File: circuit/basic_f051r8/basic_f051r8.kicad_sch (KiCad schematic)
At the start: 1 part

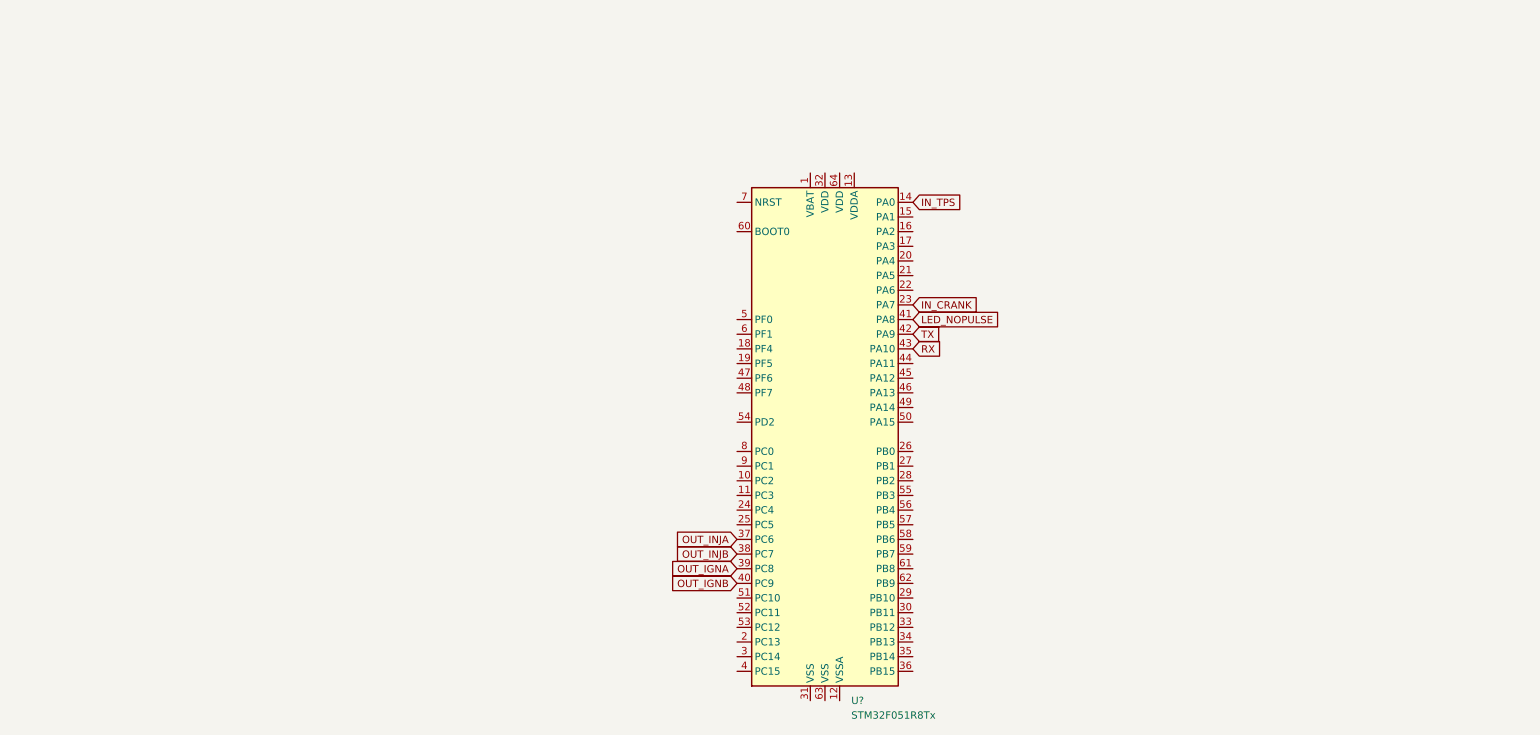
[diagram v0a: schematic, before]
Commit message: Schematic
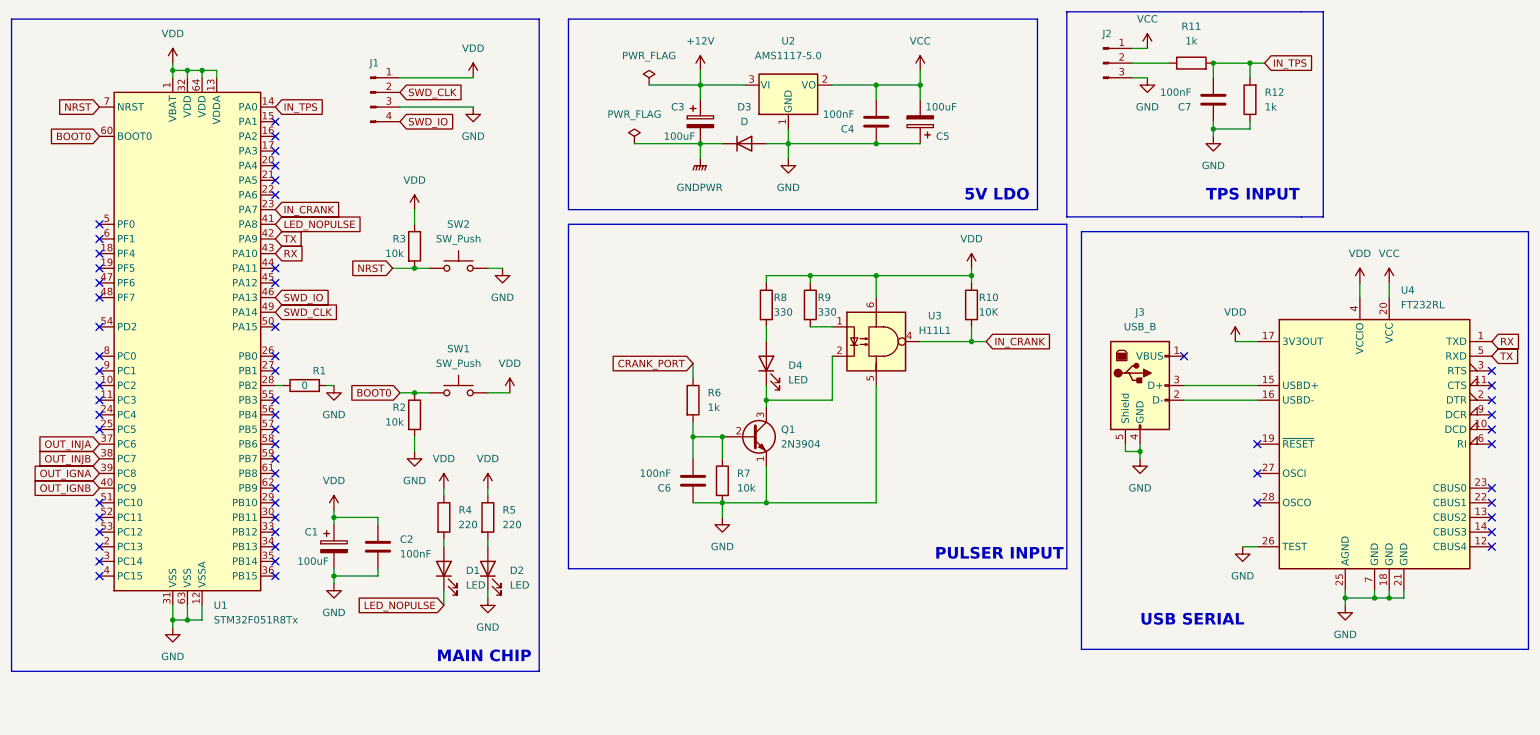
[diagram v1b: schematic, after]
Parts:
- added C1, C3, C5: 100uF, symbol Device:C_Polarized
- added C2, C4, C6, C7: 100nF, symbol Device:C
- added D1, D2, D4: LED, symbol Device:LED
- added D3: D, symbol Device:D
- added J1: Conn_01x04_Male, symbol Connector:Conn_01x04_Male
- added J2: Conn_01x03_Male, symbol Connector:Conn_01x03_Male
- added J3: USB_B, symbol Connector:USB_B
- added Q1: 2N3904, Package_TO_SOT_THT:TO-92_Inline, symbol Transistor_BJT:2N3904
- added R1: 0, symbol Device:R
- added R10: 10K, symbol Device:R
- added R11, R12, R6: 1k, symbol Device:R
- added R2, R3, R7: 10k, symbol Device:R
- added R4, R5: 220, symbol Device:R
- added R8, R9: 330, symbol Device:R
- added SW1, SW2: SW_Push, symbol Switch:SW_Push
- added U2: AMS1117-5.0, Package_TO_SOT_SMD:SOT-223-3_TabPin2, symbol Regulator_Linear:AMS1117-5.0
- added U3: H11L1, symbol Isolator:H11L1
- added U4: FT232RL, Package_SO:SSOP-28_5.3x10.2mm_P0.65mm, symbol Interface_USB:FT232RL
- gave numbers to parts that had none: 1
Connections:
- net IN_CRANK: now also R10.2, U3.4
- net IN_TPS: now also C7.2, R11.2, R12.2
- net LED_NOPULSE: now also D1.1 (K)
- net RX: now also U4.1 (TXD)
- net TX: now also U4.5 (RXD)
- net VDD: now reaches U1.1 (VBAT)
- net VDD: now also U1.13 (VDDA), U1.32 (VDD), U1.64 (VDD), C1.1, C2.1, J1.1 (Pin_1), R10.1, R3.1, R4.1, R5.1, R8.1, R9.1, SW1.2, U3.6, U4.17 (3V3OUT), U4.4 (VCCIO)
- net GND: now reaches U1.12 (VSSA)
- net GND: now also U1.31 (VSS), U1.63 (VSS), C1.2, C2.2, C4.1, C5.1, C6.1, C7.1, D2.1 (K), D3.2 (A), J1.3 (Pin_3), J2.3 (Pin_3), J3.4 (GND), J3.5 (Shield), Q1.1 (E), R1.2, R12.1, R2.2, R7.2, SW2.2, U2.1 (GND), U3.5, U4.18 (GND), U4.21 (GND), U4.25 (AGND), U4.26 (TEST), U4.7 (GND)
- net at U1.28 (PB2): now also R1.1
- net SWD_IO: now reaches U1.46 (PA13)
- net SWD_IO: now also J1.4 (Pin_4)
- net SWD_CLK: now reaches U1.49 (PA14)
- net SWD_CLK: now also J1.2 (Pin_2)
- net BOOT0: now reaches U1.60 (BOOT0)
- net BOOT0: now also R2.1, SW1.1
- net NRST: now reaches U1.7 (NRST)
- net NRST: now also R3.2, SW2.1
- new net: D4.1 (K), Q1.3 (C), U3.2
- new net: D4.2 (A), R8.2
- new net: D1.2 (A), R4.2
- new net: D2.2 (A), R5.2
- new net: C6.2, Q1.2 (B), R6.2, R7.1
- new net: J3.2 (D-), U4.16 (USBD-)
- new net: J3.3 (D+), U4.15 (USBD+)
- new net: J2.2 (Pin_2), R11.1
- new net: R9.2, U3.1
- new net +12V: C3.1, U2.3 (VI)
- new net CRANK_PORT: R6.1
- new net GNDPWR: C3.2, D3.1 (K)
- new net VCC: C4.2, C5.2, J2.1 (Pin_1), U2.2 (VO), U4.20 (VCC)
- no-connect marks 0 -> 58
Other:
- note added: "5V LDO"
- note added: "MAIN CHIP"
- note added: "PULSER INPUT"
- note added: "TPS INPUT"
- note added: "USB SERIAL"
- moved on the sheet: U1
